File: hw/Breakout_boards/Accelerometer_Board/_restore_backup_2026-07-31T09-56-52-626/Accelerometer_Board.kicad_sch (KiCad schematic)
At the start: 10 parts, among them U3 ADXL355BEZ

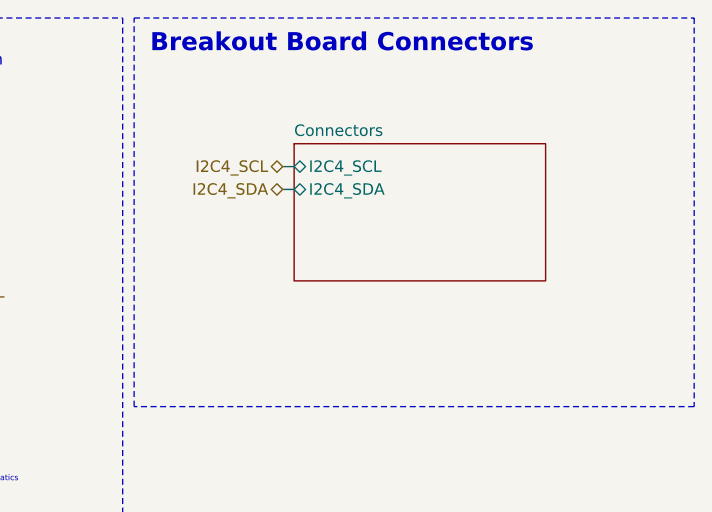
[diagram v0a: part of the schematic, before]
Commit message: Breakout Boards Measurements
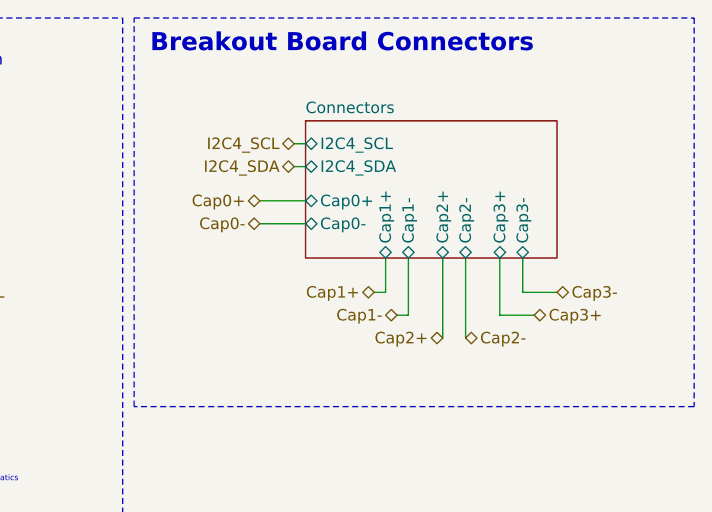
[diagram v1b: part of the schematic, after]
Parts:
- U3: footprint Acceloremeter_Analog:E_14_1-M -> ADXL355:E_14_1-M
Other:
- sheet Connectors ports: added Cap0+, Cap0-, Cap1+, Cap1-, Cap2+, Cap2-, Cap3+, Cap3-; removed none
